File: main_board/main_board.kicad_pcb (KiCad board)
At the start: 2 copper layers, 86 x 78.2 mm, 83 parts, among them J1 power, J2 debug, J3 led_matrix, J4 RJ45_LED_Shielded, J5 RJ45_LED_Shielded, J6 cathodes, J7 anodes, J8 power, Q1 BC848CWT1G, Q10 2N7002P, Q11 2N7002P, Q12 BC848CWT1G, Q13 SI2365EDS-T1-GE3, Q14 2N7002P, Q15 BC848CWT1G, Q16 2N7002P, Q17 SI2365EDS-T1-GE3, Q18 BC848CWT1G, Q19 2N7002P, Q2 SI2365EDS-T1-GE3, Q20 2N7002P, Q21 2N7002P, Q22 SI2365EDS-T1-GE3, Q23 2N7002P, Q24 BC848CWT1G, Q25 SI2365EDS-T1-GE3, Q26 CPH3350-TL-W, Q3 BC848CWT1G, Q4 2N7002P, Q5 SI2365EDS-T1-GE3, Q6 2N7002P, Q7 BC848CWT1G, Q8 SI2365EDS-T1-GE3, Q9 2N7002P, U1 AP62250, U2 Pico, U3 AP62250

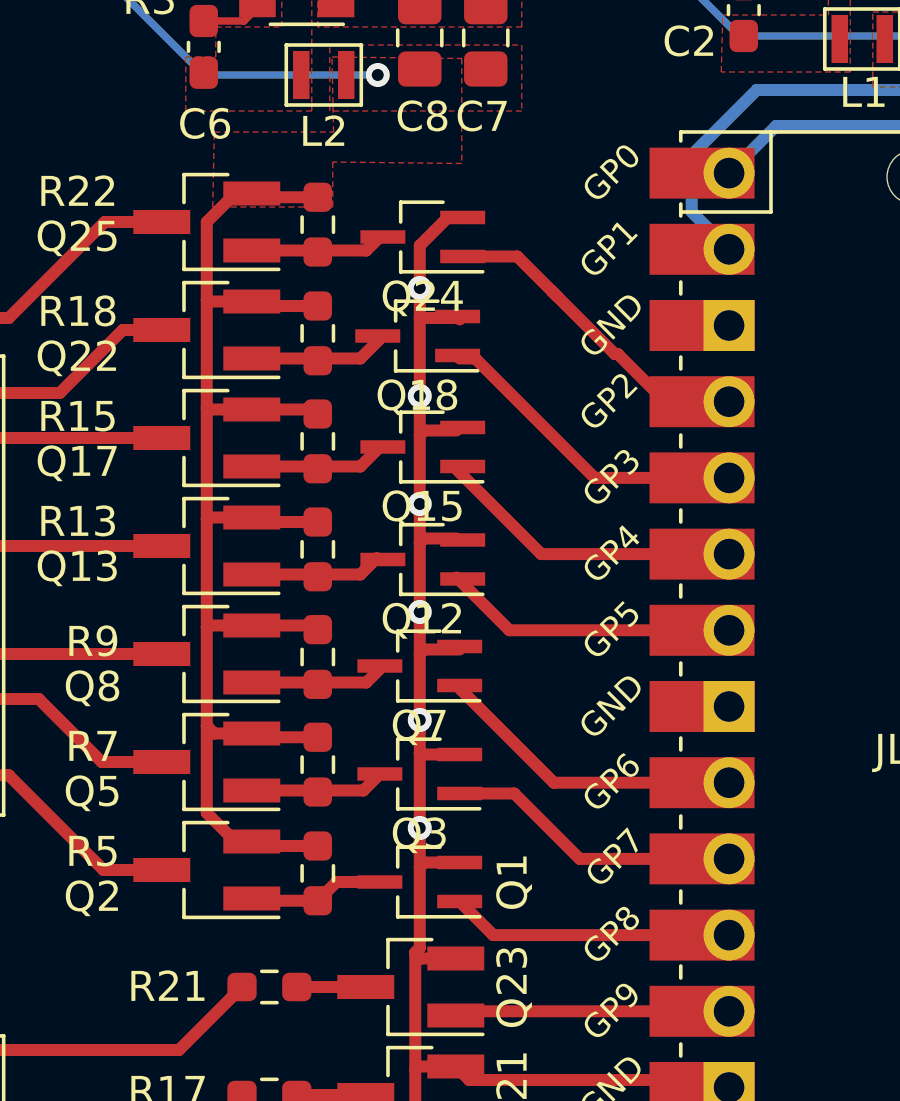
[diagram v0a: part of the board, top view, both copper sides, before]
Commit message: refactoring and segment
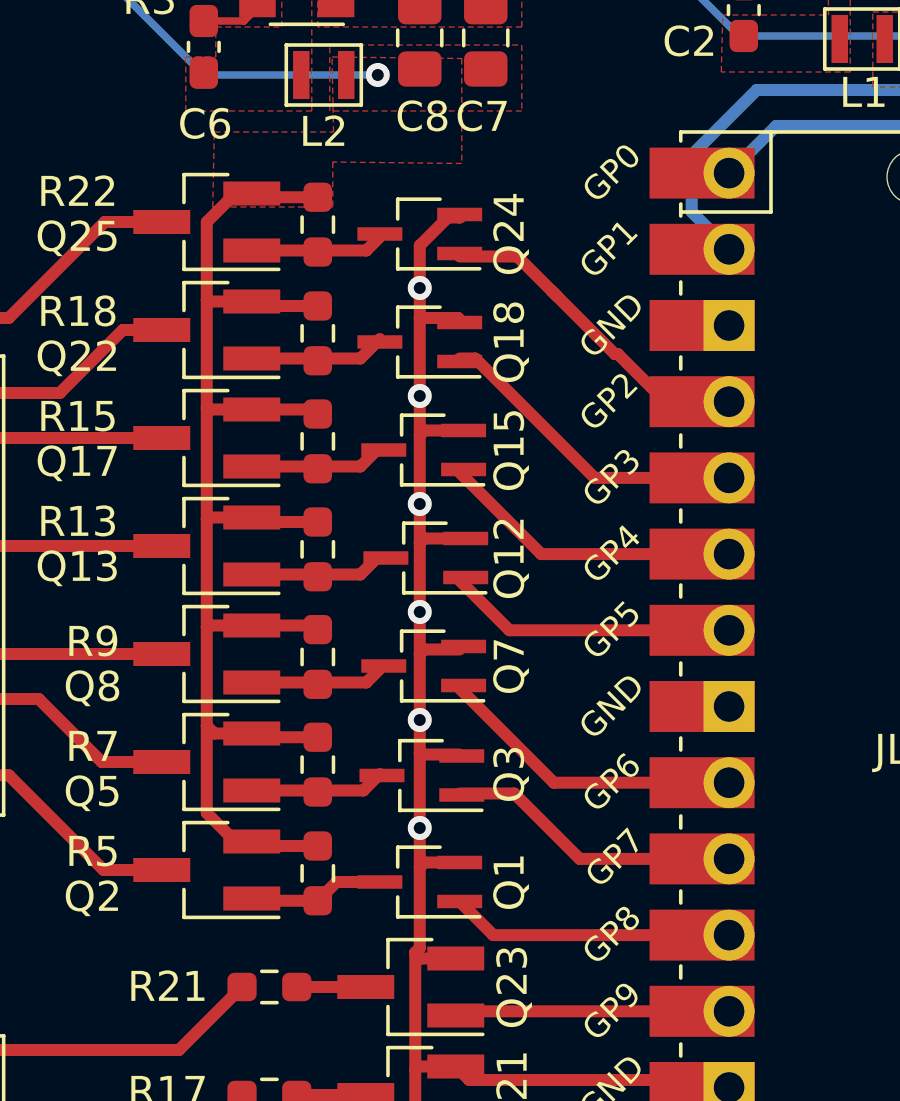
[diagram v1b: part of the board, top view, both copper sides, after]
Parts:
- Q1, Q12, Q15, Q18, Q24, Q3, Q7: value BC848CWT1G -> MCH3481-TL-W
- Q13, Q17, Q2, Q22, Q25, Q5, Q8: value SI2365EDS-T1-GE3 -> CPH3350-TL-W
- moved Q18 0.21 mm to (91.4, 81.5)
- moved Q24 0.14 mm to (91.4, 77.9)
- moved Q7 0.13 mm to (91.5, 92.3)
- moved Q12 0.11 mm to (91.6, 88.7)
- moved Q15 0.10 mm to (91.5, 85.1)
- moved Q3 0.09 mm to (91.5, 96.0)
